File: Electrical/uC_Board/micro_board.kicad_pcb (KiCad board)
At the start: 2 copper layers, 43.6 x 18 mm, 27 parts, among them J1 card_edge_6p, SW1 SW_Push, U1 ATmega328PB-AU, U2 ArdStripNano, U3 CSTNE16M0V530000R0, U4 AD8620, U5 LM1117MPX-5.0

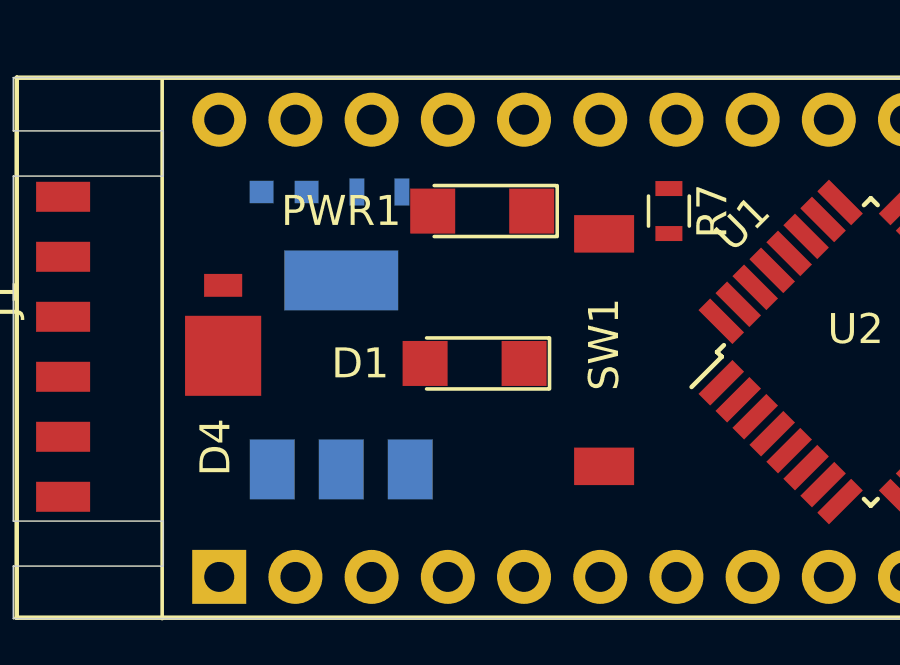
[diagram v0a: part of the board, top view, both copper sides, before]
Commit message: trying to do stuff idk
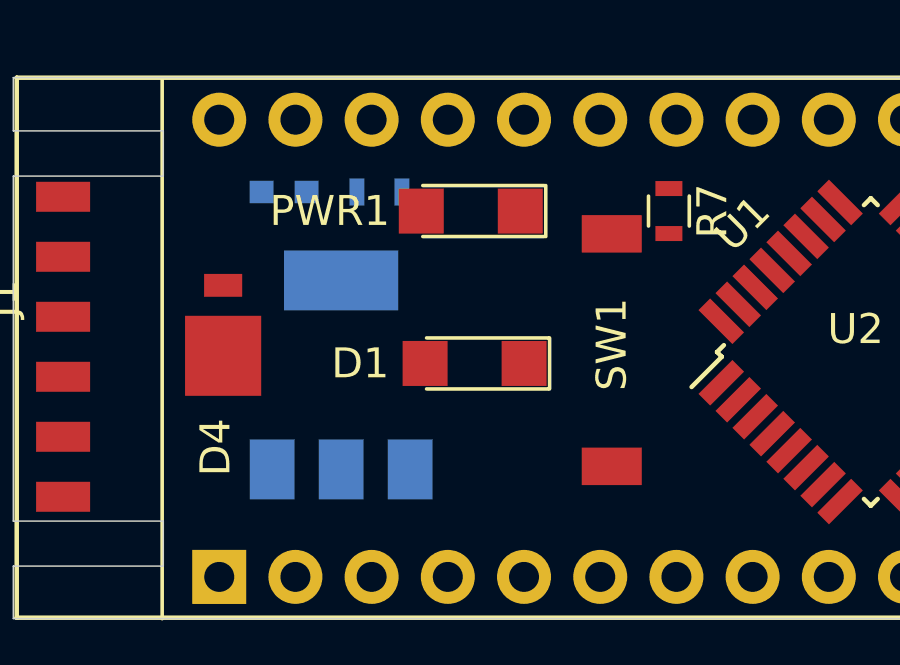
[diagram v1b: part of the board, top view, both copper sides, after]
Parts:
- moved PWR1 0.38 mm to (113.9, 106.0)
- moved SW1 0.25 mm to (118.6, 114.6)
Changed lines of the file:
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@@
   (general
     (thickness 1.6)
-    (drawings 13)
+    (drawings 14)
     (tracks 0)
     (zones 0)
@@
   )
   (module hodgkin:PTS636-G-2.5-NoGND (layer F.Cu)
-    (at 118.364 114.554 90)
+    (at 118.618 114.554 90)
     (fp_text reference SW1 (at 4.064 0 90) (layer F.SilkS)
       (effects (font (size 1 1) (thickness 0.15)))
@@
   )
   (module LEDs:LED_1206 (layer F.Cu)
-    (at 114.3 106.045 180)
+    (at 113.919 106.045 180)
     (descr "LED 1206 smd package")
     (tags "LED led 1206 SMD smd SMT smt smdled SMDLED smtled SMTLED")
@@
     )
   )
+  (gr_line (start 94.996 111.63) (end 152.146 111.63) (layer Dwgs.User) (width 0.15))
   (gr_line (start 103.632 101.6) (end 103.632 119.634) (layer F.SilkS) (width 0.12))
   (gr_line (start 142.244 101.596) (end 98.67 101.596) (layer Edge.Cuts) (width 0.05))
